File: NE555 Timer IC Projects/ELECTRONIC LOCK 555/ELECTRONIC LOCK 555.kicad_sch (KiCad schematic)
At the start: 20 parts, among them J2 Power Connector, J3 Electronic Lock, J4 Conn_02x05_Counter_Clockwise, K1 SANYOU_SRD_Form_A, Q1 AO3400A, U1 LM555xM, U2 ESP32-WROOM-32

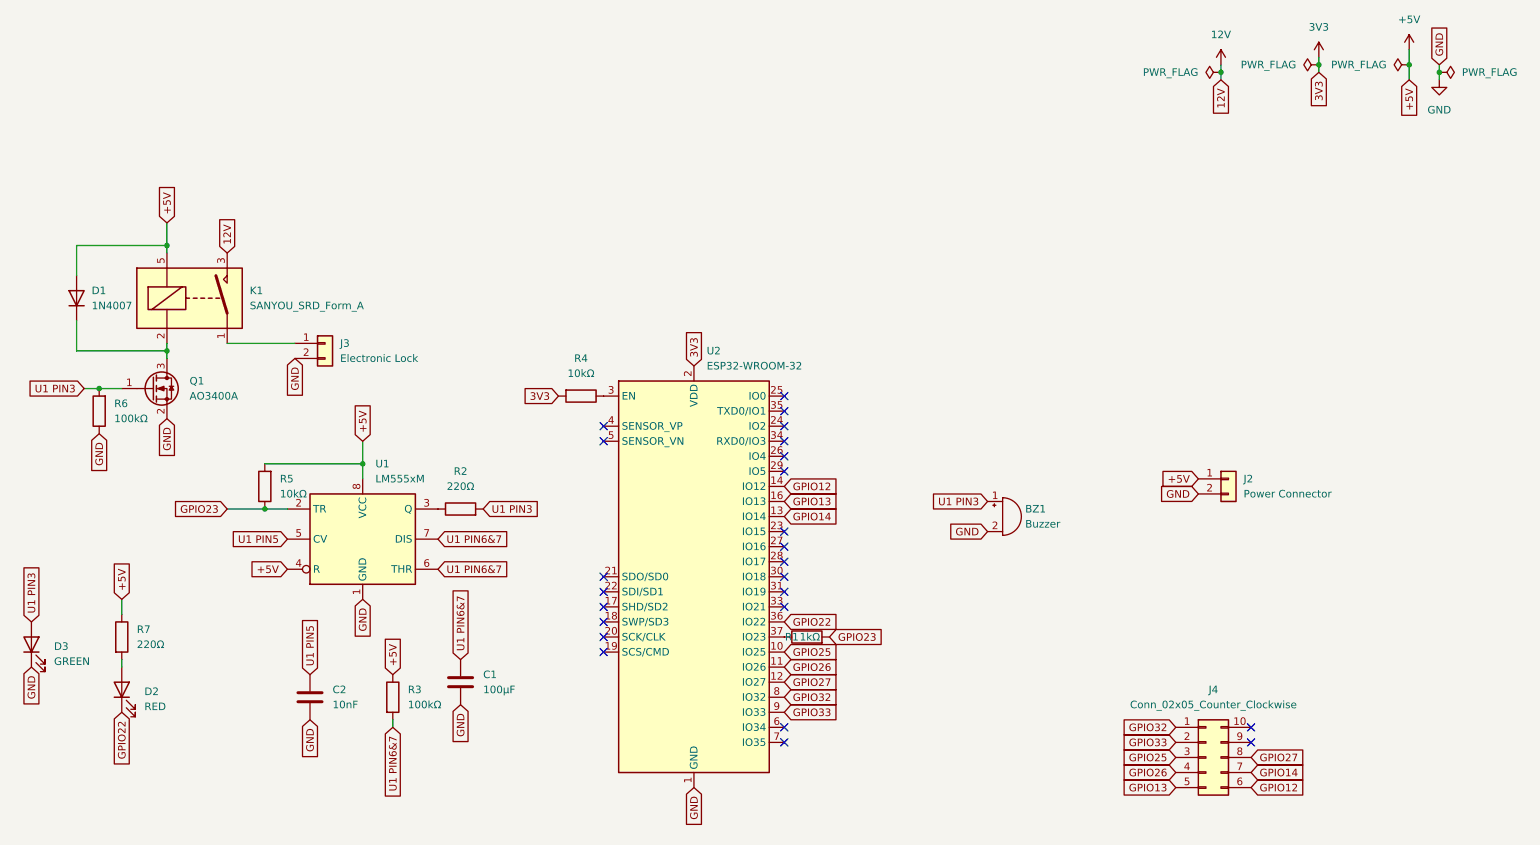
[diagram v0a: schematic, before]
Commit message: Initial Commit
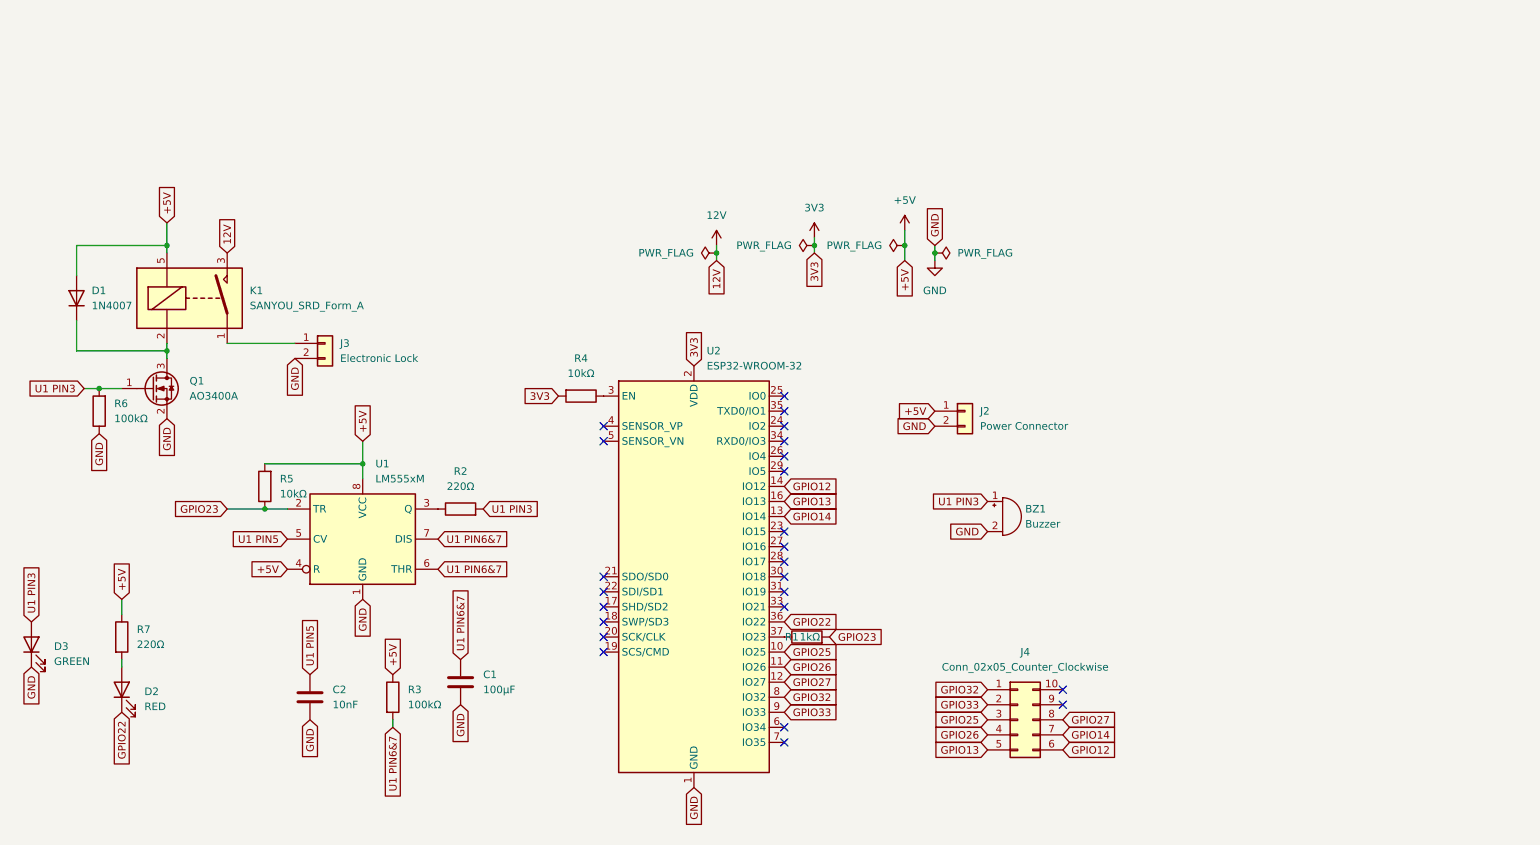
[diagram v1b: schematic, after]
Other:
- moved on the sheet: J2, J4
